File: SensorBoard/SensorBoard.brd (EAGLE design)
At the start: 134.6 x 100 mm, 75 parts, among them IC1 7805, J1 DCJ0202, U1 MPU-6000QFN-24, X1 gen1, X13 3.3out1, X14 3.3out2, X15 uart1, X16 uart2, X17 uart3, X18 uart4, X2 motordriver1, X3 MINI-USB-SCHIELD-32005-201, X4 gen2, X5 gen3, X6 gen4, X7 programmer, X8 motordriver2

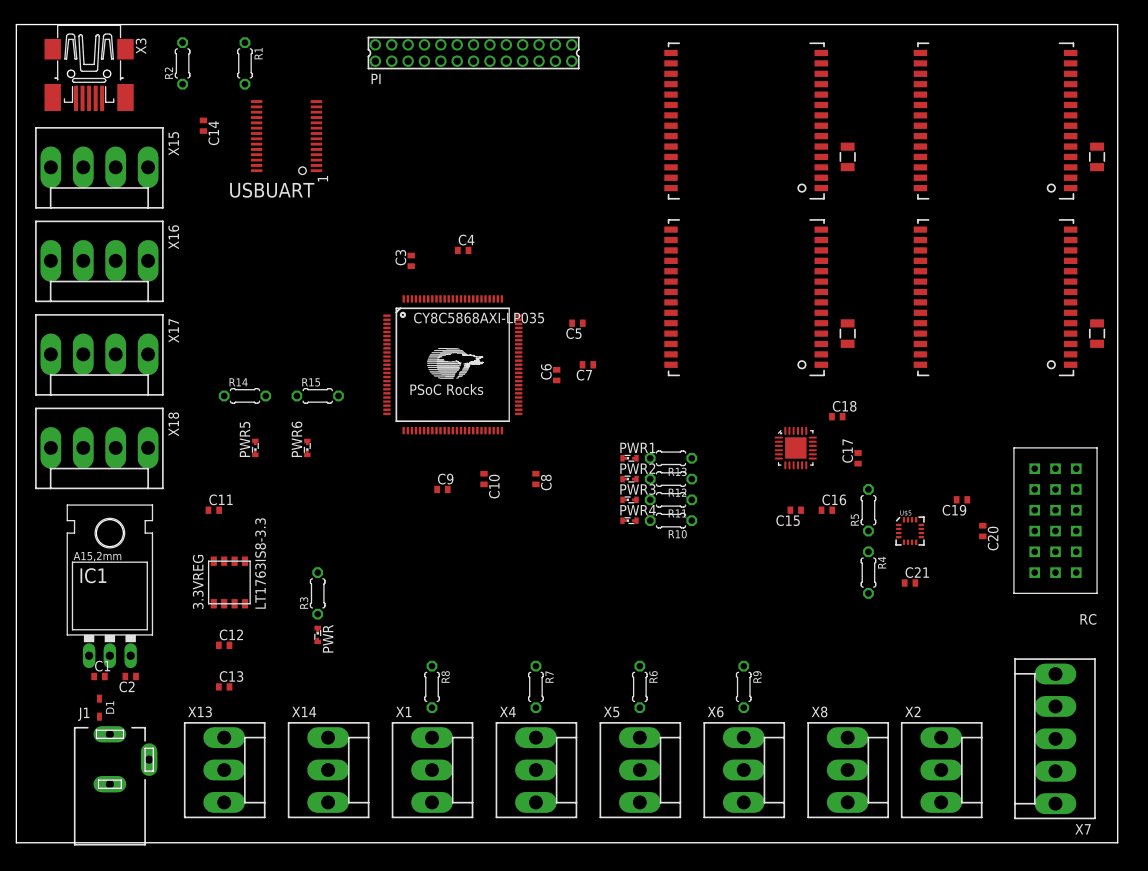
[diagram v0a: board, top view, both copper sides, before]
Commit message: fished SensorBoard.  It is perrrfect! - jack
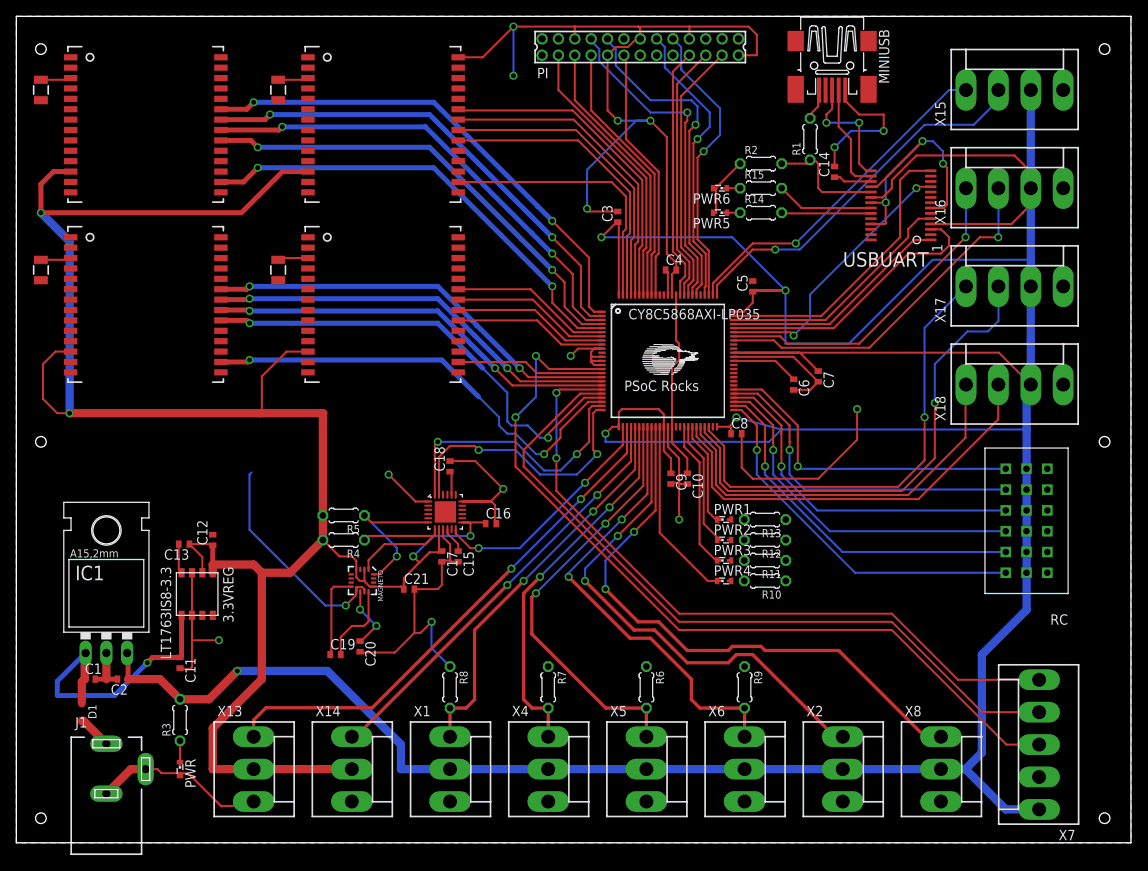
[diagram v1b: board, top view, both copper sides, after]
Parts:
- removed U$5: HMC5883LSMD, SparkFun-Sensors:16LPCC
- removed U1: MPU-6000QFN-24, SparkFun-Sensors:QFN-24-TESTING
- removed X3: MINI-USB-SCHIELD-32005-201, con-cypressindustries:32005-201
- added ACC: MPU-6000QFN-24, SparkFun-Sensors:QFN-24-TESTING
- added MAGNETO: HMC5883LSMD, SparkFun-Sensors:16LPCC
- added MINIUSB: MINI-USB-SCHIELD-32005-201, con-cypressindustries:32005-201
- moved U$2 129.3 mm to (3.00, 92.0), turned to 0 degrees
- moved X15 112.2 mm to (122.0, 92.0), turned to 0 degrees
- moved X16 112.2 mm to (122.0, 80.0), turned to 0 degrees
- moved X17 112.1 mm to (122.0, 68.0), turned to 0 degrees
- moved X18 112.1 mm to (122.0, 56.0), turned to 0 degrees
- moved U$4 104.4 mm to (32.0, 92.0), turned to 0 degrees
- moved U$1 99.6 mm to (3.00, 70.0), turned to 0 degrees
- moved GPS2 87.0 mm to (25.0, 96.0), turned to 270 degrees
- moved C19 78.9 mm to (39.0, 23.0), turned to 0 degrees
- moved C20 77.4 mm to (42.0, 24.0)
- moved C14 77.3 mm to (100.0, 82.0), turned to 90 degrees
- moved USBUART 75.6 mm to (108.1, 77.9)
- moved R2 71.7 mm to (91.0, 83.0), turned to 0 degrees
- moved U$3 70.0 mm to (32.0, 70.0), turned to 0 degrees
- moved R1 69.7 mm to (97.0, 86.0), turned to 90 degrees
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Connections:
- new net +3.3VP1: PI.1
- new net +3.3VP2: PI.17
- new net +5VP1: PI.2
- new net +5VP2: PI.4
- new net 1: CY8C5868AXI-LP035.90
- new net 2: CY8C5868AXI-LP035.89
- new net 3: CY8C5868AXI-LP035.80
- new net 37: CY8C5868AXI-LP035.49
- new net 44: CY8C5868AXI-LP035.67
- net +3.3V: now also ACC.13, ACC.8, MAGNETO.13, MAGNETO.2, MAGNETO.4; no longer PI.1, PI.17, U$5.13, U$5.2, U$5.4, U1.13, U1.8
- net +5V: no longer PI.2, PI.4
- net AUXCL1: now also ACC.7, MAGNETO.1; no longer U$5.1, U1.7
- net AUXDA1: now also ACC.6, MAGNETO.16; no longer U$5.16, U1.6
- net CH1: now also CY8C5868AXI-LP035.51; no longer CY8C5868AXI-LP035.42
- net CH2: now also CY8C5868AXI-LP035.52; no longer CY8C5868AXI-LP035.43
- net CH3: now also CY8C5868AXI-LP035.53; no longer CY8C5868AXI-LP035.44
- net CH4: now also CY8C5868AXI-LP035.54; no longer CY8C5868AXI-LP035.47
- net CH5: now also CY8C5868AXI-LP035.55; no longer CY8C5868AXI-LP035.48
- net CH6: now also CY8C5868AXI-LP035.56; no longer CY8C5868AXI-LP035.49
- net CLKOUT1: now also ACC.22; no longer U1.22
- net CTS#: now also CY8C5868AXI-LP035.70; no longer CY8C5868AXI-LP035.36
- net D+: now also MINIUSB.3; no longer X3.3
- net D-: now also MINIUSB.2; no longer X3.2
- net FSYNC: now also ACC.11; no longer U1.11
- net GEN1: now also CY8C5868AXI-LP035.30; no longer CY8C5868AXI-LP035.31
- net GEN2: now also CY8C5868AXI-LP035.31; no longer CY8C5868AXI-LP035.32
- net GEN3: now also CY8C5868AXI-LP035.32; no longer CY8C5868AXI-LP035.33
- net GEN4: now also CY8C5868AXI-LP035.33; no longer CY8C5868AXI-LP035.34
- net GEN5: now also CY8C5868AXI-LP035.28; no longer CY8C5868AXI-LP035.29
- net GEN6: now also CY8C5868AXI-LP035.29; no longer CY8C5868AXI-LP035.30
- net GND: now also ACC.1, ACC.18, ACC.9, MAGNETO.11, MAGNETO.9, MINIUSB.1; no longer U$5.11, U$5.9, U1.1, U1.18, U1.9, X3.1
- net GPIO10: now also CY8C5868AXI-LP035.85; no longer CY8C5868AXI-LP035.82
- net GPIO11: now also CY8C5868AXI-LP035.83; no longer CY8C5868AXI-LP035.80
- net GPIO14: now also CY8C5868AXI-LP035.82; no longer CY8C5868AXI-LP035.1
- net GPIO15: now also CY8C5868AXI-LP035.81; no longer CY8C5868AXI-LP035.2
- net GPIO17: now also CY8C5868AXI-LP035.91; no longer CY8C5868AXI-LP035.85
- net GPIO18: no longer CY8C5868AXI-LP035.3
- net GPIO2(0): now also CY8C5868AXI-LP035.94; no longer CY8C5868AXI-LP035.91
- net GPIO22: no longer CY8C5868AXI-LP035.83
- net GPIO23: now also CY8C5868AXI-LP035.79; no longer CY8C5868AXI-LP035.16
- net GPIO24: now also CY8C5868AXI-LP035.78; no longer CY8C5868AXI-LP035.17
- net GPIO25: no longer CY8C5868AXI-LP035.18
- net GPIO27: no longer CY8C5868AXI-LP035.84
- net GPIO3(1): now also CY8C5868AXI-LP035.93; no longer CY8C5868AXI-LP035.90
- net GPIO4: now also CY8C5868AXI-LP035.92; no longer CY8C5868AXI-LP035.89
- net GPIO7: no longer CY8C5868AXI-LP035.52
- net GPIO8: no longer CY8C5868AXI-LP035.19
- net GPIO9: now also CY8C5868AXI-LP035.84; no longer CY8C5868AXI-LP035.81
- net GPS1RXA: now also CY8C5868AXI-LP035.19; no longer CY8C5868AXI-LP035.7
- net GPS1RXB: now also CY8C5868AXI-LP035.22; no longer CY8C5868AXI-LP035.9
- net GPS1TXA: now also CY8C5868AXI-LP035.17; no longer CY8C5868AXI-LP035.6
- net GPS1TXB: now also CY8C5868AXI-LP035.18; no longer CY8C5868AXI-LP035.8
- net GPS1XSTB: now also CY8C5868AXI-LP035.23; no longer CY8C5868AXI-LP035.22
- net GPS2RXA: now also CY8C5868AXI-LP035.3; no longer CY8C5868AXI-LP035.98
- net GPS2RXB: now also CY8C5868AXI-LP035.4; no longer CY8C5868AXI-LP035.96
- net GPS2TXA: now also CY8C5868AXI-LP035.1; no longer CY8C5868AXI-LP035.99
- net GPS2TXB: now also CY8C5868AXI-LP035.2; no longer CY8C5868AXI-LP035.97
- net GPS2XSTB: now also CY8C5868AXI-LP035.5; no longer CY8C5868AXI-LP035.23
- net GPS3RXA: now also CY8C5868AXI-LP035.8; no longer CY8C5868AXI-LP035.94
- net GPS3RXB: now also CY8C5868AXI-LP035.9; no longer CY8C5868AXI-LP035.92
- net GPS3TXA: now also CY8C5868AXI-LP035.6; no longer CY8C5868AXI-LP035.95
- net GPS3TXB: now also CY8C5868AXI-LP035.7; no longer CY8C5868AXI-LP035.93
- net GPS3XSTB: now also CY8C5868AXI-LP035.16; no longer CY8C5868AXI-LP035.24
- net GPS4RXA: now also CY8C5868AXI-LP035.97; no longer CY8C5868AXI-LP035.78
- net GPS4RXB: now also CY8C5868AXI-LP035.98; no longer CY8C5868AXI-LP035.76
- net GPS4TXA: now also CY8C5868AXI-LP035.95; no longer CY8C5868AXI-LP035.79
- net GPS4TXB: now also CY8C5868AXI-LP035.96; no longer CY8C5868AXI-LP035.77
- net GPS4XSTB: now also CY8C5868AXI-LP035.99; no longer CY8C5868AXI-LP035.25
- net INT1: now also ACC.12, CY8C5868AXI-LP035.27; no longer U1.12
- net MDTX1: now also CY8C5868AXI-LP035.34; no longer CY8C5868AXI-LP035.46
- net MDTX2: now also CY8C5868AXI-LP035.35; no longer CY8C5868AXI-LP035.45
- net N$11: now also MAGNETO.12; no longer U$5.12
- net N$15: now also MAGNETO.8; no longer U$5.8
- net N$16: now also MAGNETO.10; no longer U$5.10
- net N$6: now also MINIUSB.4, MINIUSB.5; no longer X3.4, X3.5
- net N$7: now also ACC.10; no longer U1.10
- net N$8: now also ACC.20; no longer U1.20
- net PWREN#: now also CY8C5868AXI-LP035.74
- net RTS#: now also CY8C5868AXI-LP035.71; no longer CY8C5868AXI-LP035.35
- net RX1: now also CY8C5868AXI-LP035.77; no longer CY8C5868AXI-LP035.74
- net RX2: now also CY8C5868AXI-LP035.69; no longer CY8C5868AXI-LP035.72
- net RX3: now also CY8C5868AXI-LP035.48; no longer CY8C5868AXI-LP035.70
- net RX4: now also CY8C5868AXI-LP035.46; no longer CY8C5868AXI-LP035.68
- net SCL_ACC: now also ACC.23, CY8C5868AXI-LP035.25; no longer CY8C5868AXI-LP035.4, U1.23
- net SDA_ACC: now also ACC.24, CY8C5868AXI-LP035.24; no longer CY8C5868AXI-LP035.5, U1.24
- net STATUS1: now also CY8C5868AXI-LP035.44; no longer CY8C5868AXI-LP035.56
- net STATUS2: now also CY8C5868AXI-LP035.43; no longer CY8C5868AXI-LP035.55
- net STATUS3: now also CY8C5868AXI-LP035.42; no longer CY8C5868AXI-LP035.54
- net STATUS4: now also CY8C5868AXI-LP035.36; no longer CY8C5868AXI-LP035.53
- net TX1: now also CY8C5868AXI-LP035.76; no longer CY8C5868AXI-LP035.73
- net TX2: now also CY8C5868AXI-LP035.68; no longer CY8C5868AXI-LP035.71
- net TX3: now also CY8C5868AXI-LP035.47; no longer CY8C5868AXI-LP035.69
- net TX4: now also CY8C5868AXI-LP035.45; no longer CY8C5868AXI-LP035.67
- net USB_RXD: now also CY8C5868AXI-LP035.73; no longer CY8C5868AXI-LP035.27
- net USB_TXD: now also CY8C5868AXI-LP035.72; no longer CY8C5868AXI-LP035.28
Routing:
- net +5V: track 0.00 -> 475.9 mm, vias 0 -> 5
- net GND: track 0.00 -> 371.4 mm, vias 0 -> 18
- net +3.3V: track 0.00 -> 247.9 mm, vias 0 -> 4
- net XRES: track 0.00 -> 101.4 mm, vias 0 -> 2
- net SCLK: track 0.00 -> 89.9 mm
- net SDAT: track 0.00 -> 86.3 mm, vias 0 -> 2
- net MDTX2: track 0.00 -> 71.3 mm, vias 0 -> 2
- net GEN5: track 0.00 -> 64.4 mm, vias 0 -> 2
- net MDTX1: track 0.00 -> 62.4 mm, vias 0 -> 2
- net TX3: track 0.00 -> 61.6 mm, vias 0 -> 1
- net GPS2TXA: track 0.00 -> 61.0 mm, vias 0 -> 2
- net GPS2TXB: track 0.00 -> 60.0 mm, vias 0 -> 2
- net GPS2RXA: track 0.00 -> 58.9 mm, vias 0 -> 2
- net GPS2RXB: track 0.00 -> 57.6 mm, vias 0 -> 2
- net GPS1RXB: track 0.00 -> 56.9 mm, vias 0 -> 2
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- added copper zone on layer 1, net GND
- added copper zone on layer 16, net GND
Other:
- board size 134.6 x 100 mm -> 136.2 x 101 mm
